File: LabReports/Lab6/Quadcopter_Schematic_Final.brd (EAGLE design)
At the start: 100.3 x 100.3 mm, 53 parts, among them J1 AVR_SPI_PRG_6NS, U1 ATMEGA128RFA1, Y1 16MHz

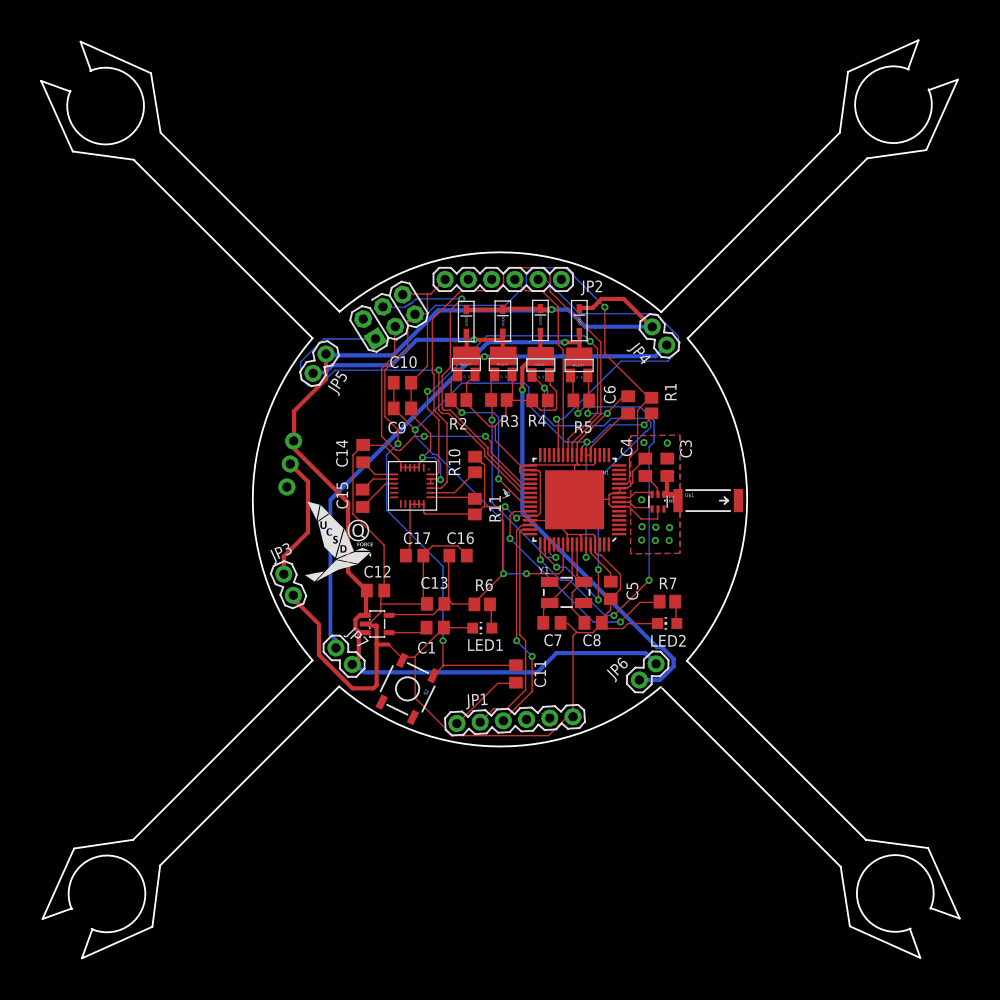
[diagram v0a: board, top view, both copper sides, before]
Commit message: board layout
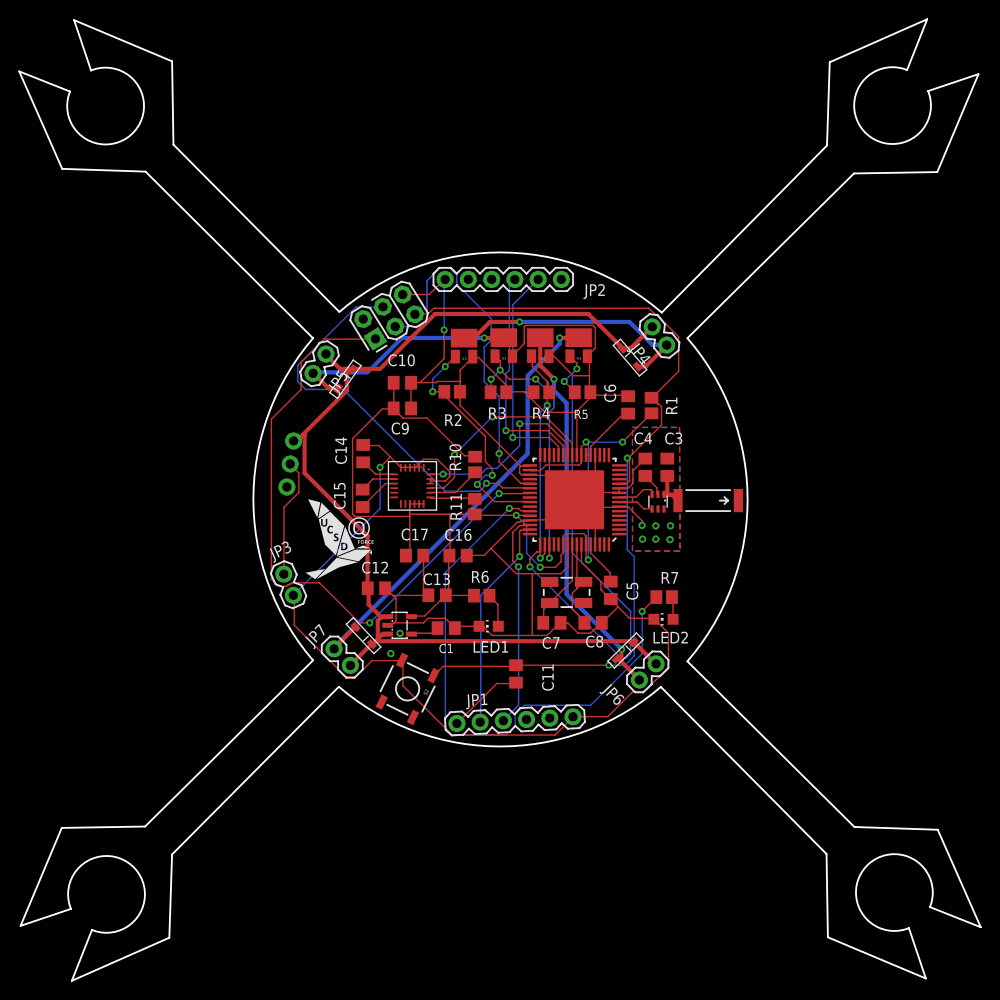
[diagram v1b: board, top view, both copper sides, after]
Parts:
- U$11: device Andranik-Lab4:LOGOS -> Andranik-Lab4:LOGOSBOTTOM
- U$12: device Andranik-Lab4:LOGOSBOTTOM -> Andranik-Lab4:LOGOS
- moved U$10 41.7 mm to (-14.9, -14.9), turned to 133.2 degrees
- moved U$8 37.2 mm to (13.7, -16.5), turned to 224.6 degrees
- moved U$6 18.4 mm to (-16.9, 13.1), turned to 234.1 degrees
- moved U$4 18.3 mm to (14.2, 15.5), turned to 310.7 degrees
- moved U$12 11.8 mm to (-22.9, -9.35)
- moved U$11 10.5 mm to (-19.1, -19.4)
- moved U$2 2.45 mm to (-11.0, -13.8)
- moved U$9 2.10 mm to (8.57, 15.8)
- moved U$7 2.05 mm to (4.38, 15.8)
- moved U$5 2.00 mm to (0.39, 15.8)
- moved U$3 1.97 mm to (-3.95, 15.8)
- moved C1 1.20 mm to (-5.90, -14.1)
- moved R2 1.14 mm to (-5.25, 11.8)
- moved C13 0.96 mm to (-6.90, -10.5)
- moved R6 0.95 mm to (-2.02, -10.5)
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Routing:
- net GND: track 270.0 -> 324.9 mm, vias 13 -> 8
- net SCL: track 59.9 -> 22.7 mm, vias 0 -> 2
- net PB7: track 25.9 -> 62.3 mm
- net 3V: track 146.7 -> 119.3 mm, vias 8 -> 5
- net MISO: track 45.6 -> 70.6 mm, vias 1 -> 2
- net SDA: track 45.3 -> 20.8 mm
- net PE4: track 50.0 -> 26.1 mm, vias 4 -> 2
- net POWER: track 133.3 -> 115.8 mm, vias 1 -> 0
- net TX1: track 39.9 -> 24.7 mm
- net MOSI: track 35.5 -> 44.7 mm
- net PE3: track 49.1 -> 57.0 mm, vias 4 -> 3
- net N$33: track 49.4 -> 42.5 mm, vias 1 -> 2
- net SCK: track 32.9 -> 39.4 mm, vias 2 -> 1
- net RESET: track 101.8 -> 95.6 mm, vias 3 -> 2
- net PB5: track 20.4 -> 26.3 mm, vias 2 -> 4
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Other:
- board size 100.3 x 100.3 mm -> 105 x 105.1 mm
- board text removed: "C:/Users/Andranik/Desktop/LOGOQUAD.bmp"
